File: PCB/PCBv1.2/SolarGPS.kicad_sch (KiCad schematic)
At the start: 58 parts, among them J1 Conn_01x10_Female, J2 Solar1+, J3 GND, J4 Conn_02x03_Odd_Even, J5 Solar2+, J6 GND, J7 Screw_Terminal_01x01, J8 Conn_01x04_Male, U1 STM32L011G3Ux, U2 MAX-M10Q, U5 BQ25505, U6 LIS3DH, U7 TPS63802, Y1 32.768

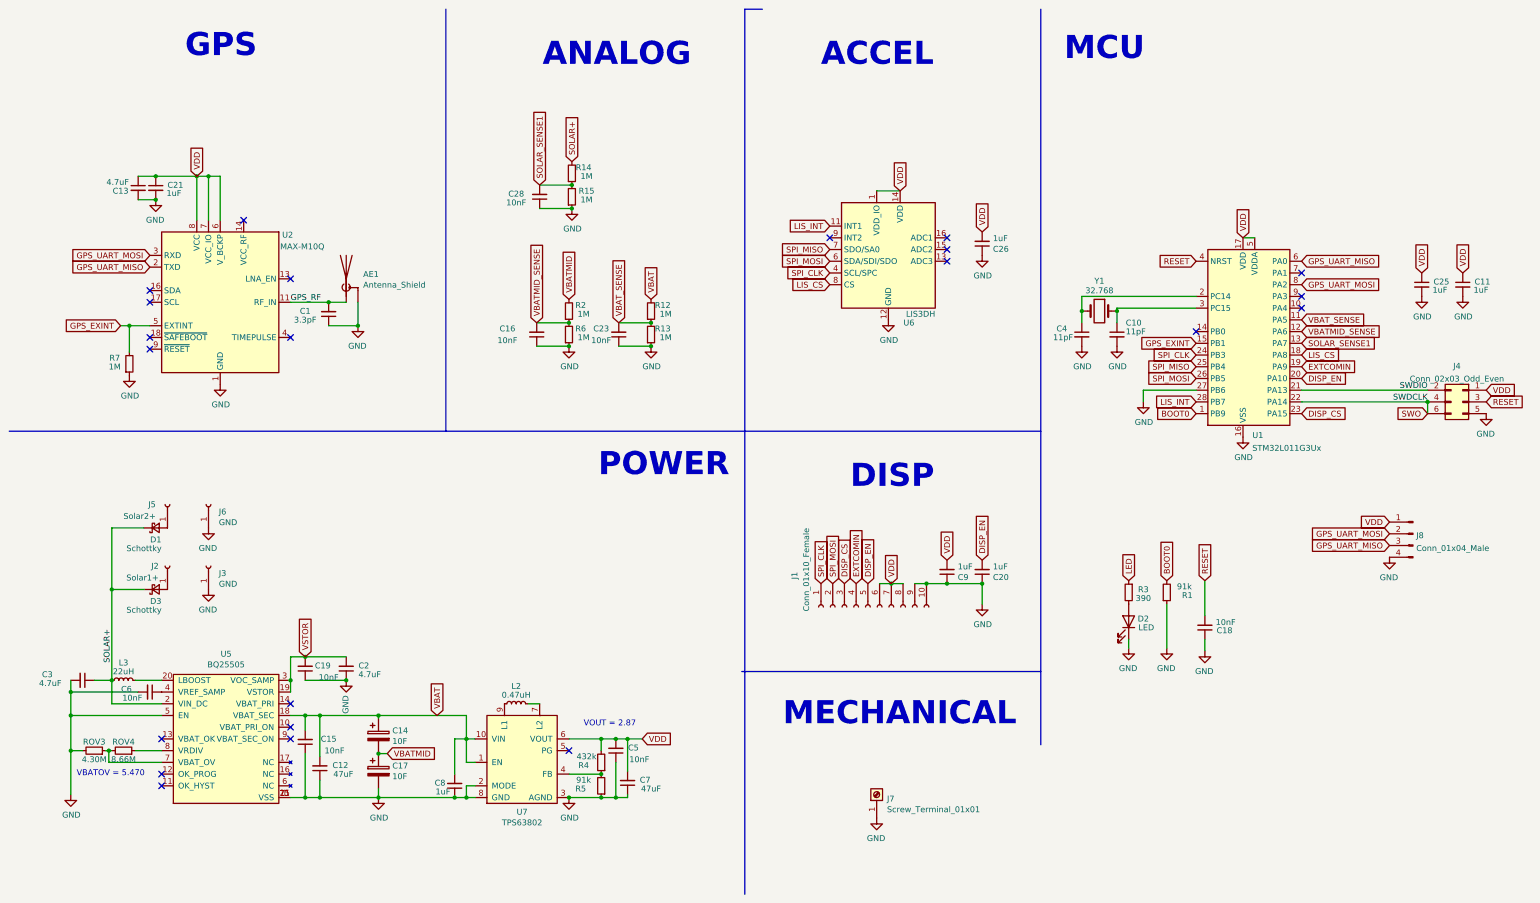
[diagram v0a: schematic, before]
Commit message: Rebuild PCB1.2 and submit for build
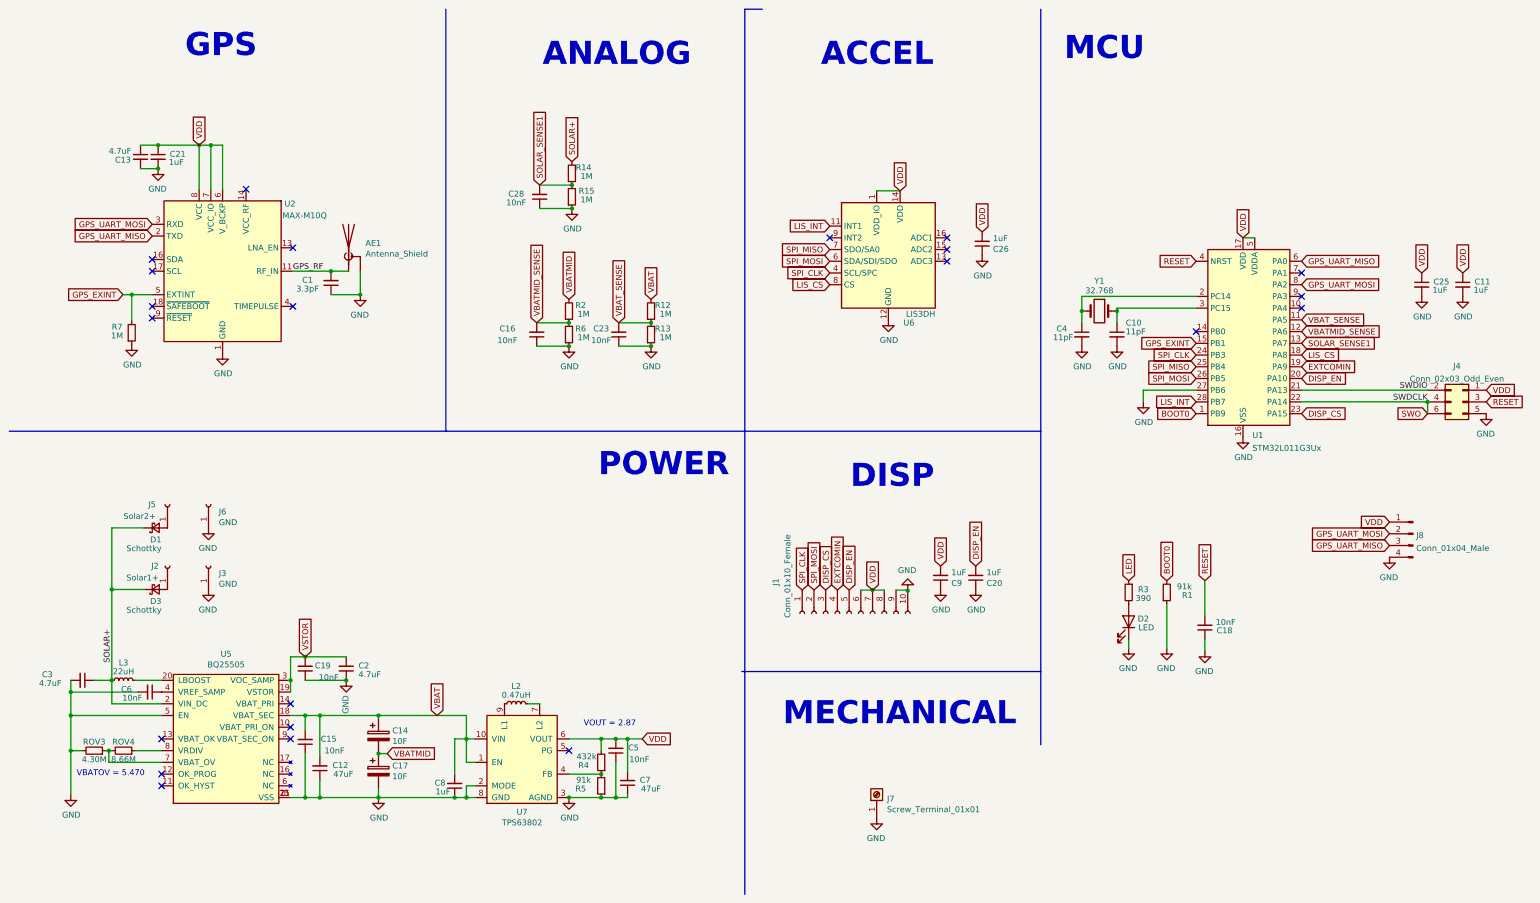
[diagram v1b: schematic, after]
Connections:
- net GND: no longer J1.10 (Pin_10), J1.9 (Pin_9)
- new net: J1.10 (Pin_10), J1.9 (Pin_9)
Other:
- moved on the sheet: AE1, C1, C13, C20, C21, C9, J1, R7, U2
